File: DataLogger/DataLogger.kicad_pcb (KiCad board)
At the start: 2 copper layers, 76 x 69.6 mm, 33 parts, among them J1 UART, J2 SPI, J3 I2C, J4 Battery, J5 Conn_01x06_Pin, J6 Conn_01x04_Pin, SW1 SW_Push, SW2 SW_SPDT, U1 ATmega328-P, U2 24LC1025, U3 DS1337, U4 24LC1025, Y1 Crystal, Y2 Crystal

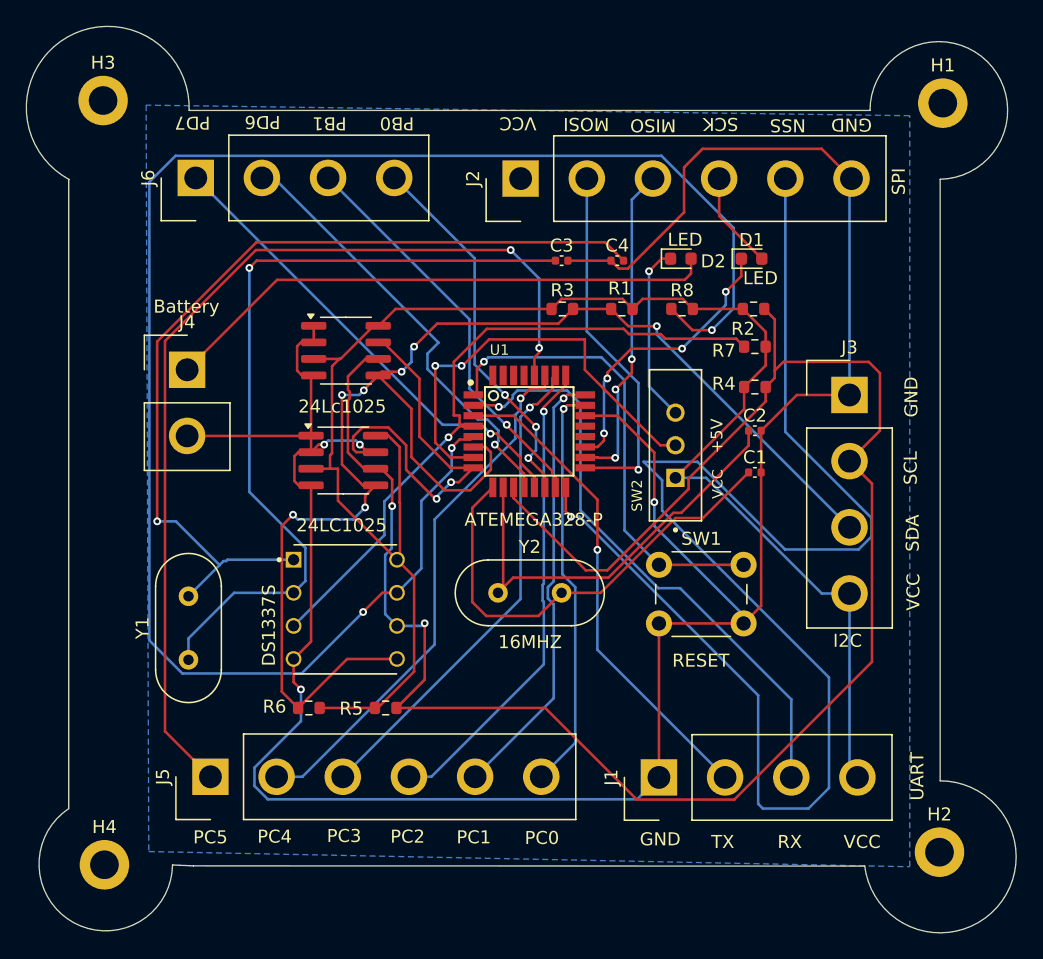
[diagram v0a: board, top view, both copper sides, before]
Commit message: edited new tracks
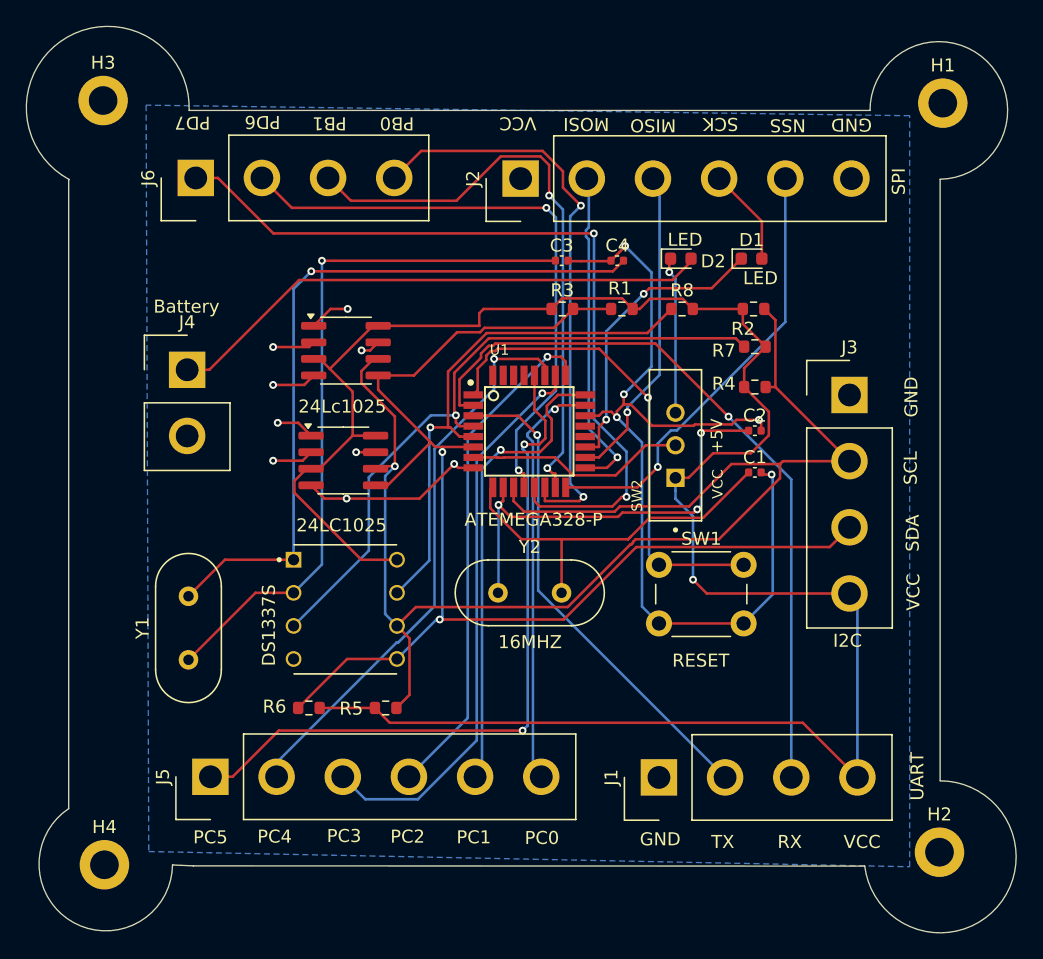
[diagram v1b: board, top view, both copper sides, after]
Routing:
- net GND: track 230.0 -> 104.9 mm, vias 6 -> 14
- net /INTB: track 133.0 -> 40.8 mm, vias 3 -> 1
- net NSS: track 118.9 -> 34.2 mm
- net /SCL: track 147.1 -> 110.8 mm, vias 2 -> 1
- net /VCC: track 132.3 -> 160.6 mm, vias 0 -> 1
- net Net-(J6-Pin_1): track 36.6 -> 62.2 mm, vias 1 -> 2
- net Net-(J5-Pin_1): track 75.0 -> 54.8 mm
- net +5V: track 33.3 -> 17.1 mm, vias 2 -> 0
- net Net-(J6-Pin_4): track 29.0 -> 44.9 mm, vias 3 -> 2
- net Net-(J6-Pin_3): track 31.0 -> 45.4 mm, vias 1 -> 2
- net Net-(U3-X1): track 68.8 -> 56.2 mm
- net Net-(J6-Pin_2): track 34.0 -> 46.2 mm, vias 1 -> 2
- net /SDA: track 109.1 -> 97.2 mm, vias 7 -> 2
- net /RX: track 45.7 -> 57.1 mm
- net Net-(U3-X2): track 62.0 -> 54.5 mm
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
